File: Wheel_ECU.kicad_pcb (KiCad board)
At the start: 2 copper layers, 61 x 61 mm, 64 parts, among them J1 Conn_01x04, J2 Conn_01x04, J3 Conn_01x02, J4 Debug, J5 Conn_01x02, U1 IFX9201SG, U2 TLE4964, U3 XMC1404_F064, U4 TLE7251, U5 LM35-D

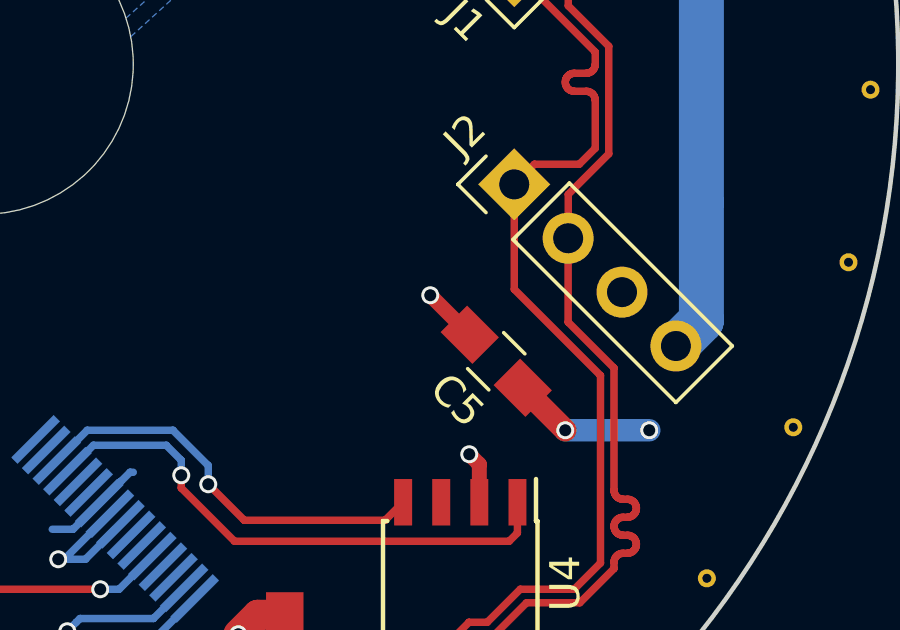
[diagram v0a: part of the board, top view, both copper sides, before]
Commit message: Smaller clean up
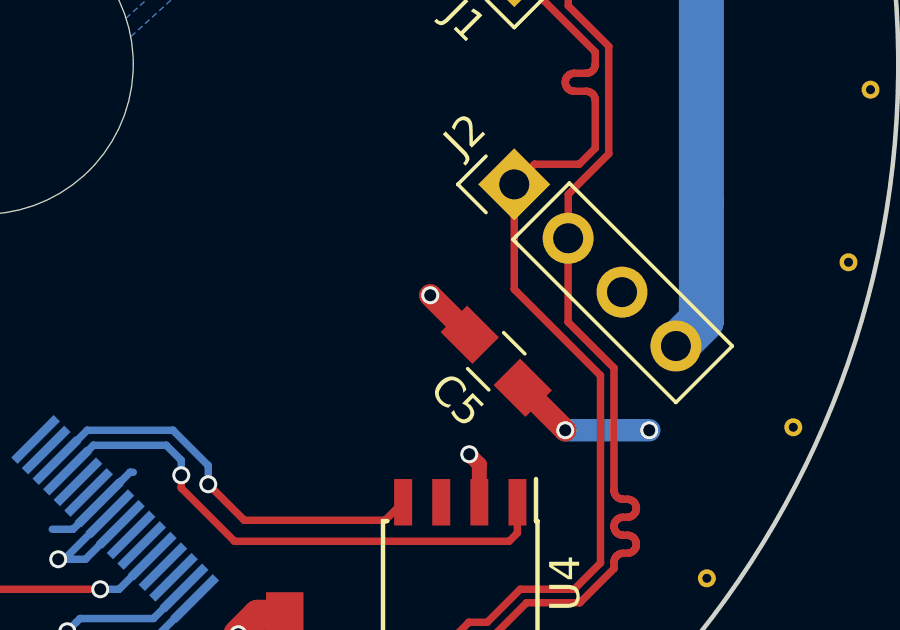
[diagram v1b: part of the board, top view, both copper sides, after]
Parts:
- moved G*** 0.23 mm to (113.1, 81.5)
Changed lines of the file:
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@@
   )
   (setup
-    (last_trace_width 1)
+    (last_trace_width 0.75)
     (user_trace_width 0.35)
     (user_trace_width 0.5)
@@
   )
   (module WheelECU:Logo_Wolley_Interconnect_SolderMask (layer F.Cu)
-    (at 113.03 81.28)
+    (at 113.1 81.5)
     (fp_text reference G*** (at 0 0) (layer F.SilkS) hide
       (effects (font (size 1.524 1.524) (thickness 0.3)))
@@
   (segment (start 135.666116 113.02642) (end 136.692536 112) (width 0.25) (layer B.Cu) (net 1))
   (segment (start 136.692536 112) (end 136.8 112) (width 0.25) (layer B.Cu) (net 1))
-  (segment (start 148.016117 107.416117) (end 146.7 106.1) (width 0.5) (layer F.Cu) (net 1))
   (via (at 146.7 106.1) (size 0.6) (drill 0.4) (layers F.Cu B.Cu) (net 1))
   (segment (start 151.8 85.4) (end 145.696051 85.403949) (width 1.5) (layer B.Cu) (net 1))
@@
   (segment (start 131.7 81.9) (end 128.6 78.8) (width 0.75) (layer F.Cu) (net 1))
   (segment (start 131.7 82.5) (end 131.7 81.9) (width 0.75) (layer F.Cu) (net 1))
+  (segment (start 148.016117 107.416117) (end 146.7 106.1) (width 0.75) (layer F.Cu) (net 1))
   (segment (start 151.2 110.6) (end 154 110.6) (width 0.75) (layer B.Cu) (net 2))
   (via (at 154 110.6) (size 0.6) (drill 0.4) (layers F.Cu B.Cu) (net 2))
